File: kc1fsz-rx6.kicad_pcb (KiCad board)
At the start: 2 copper layers, 63.5 x 47.8 mm, 51 parts, among them J1 Conn_Coaxial, J2 Conn_01x07, J3 Conn_01x02, J4 Conn_01x02, U1 SN74CBT3253, U2 LM4562, U3 LM4562

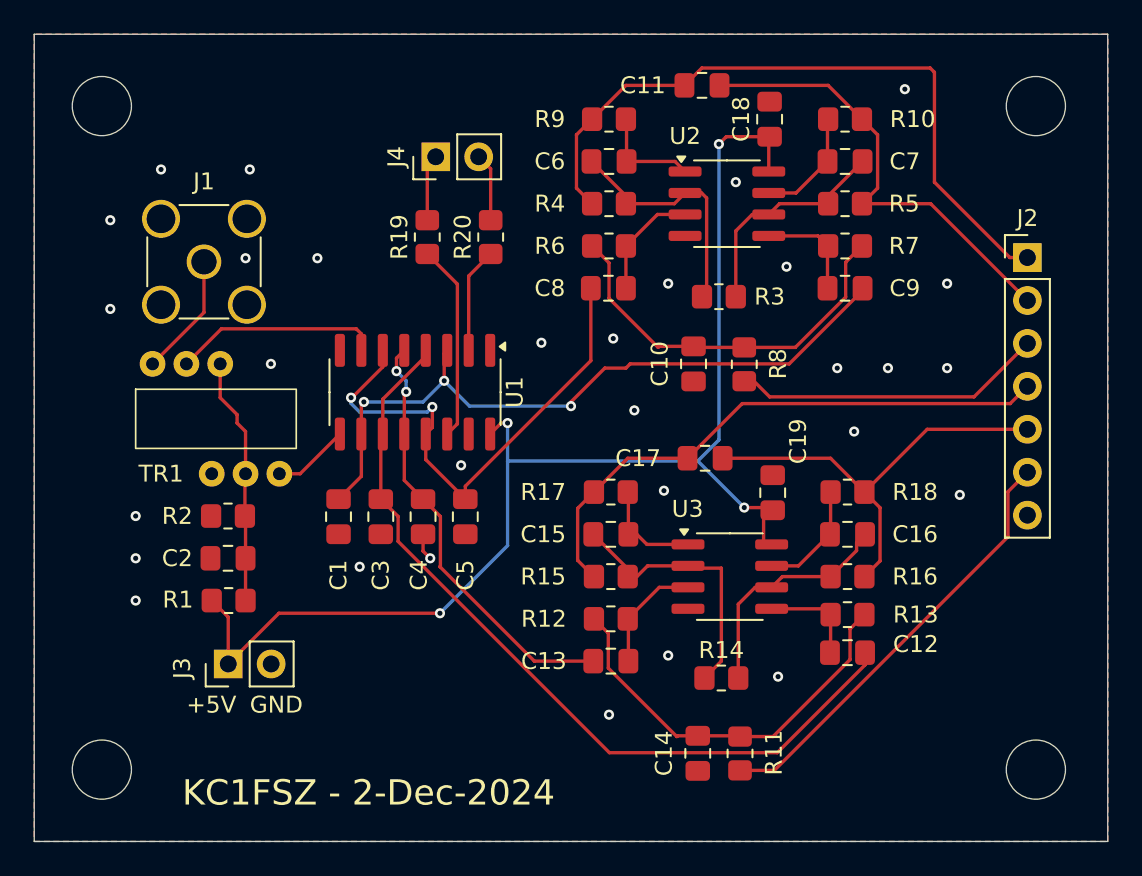
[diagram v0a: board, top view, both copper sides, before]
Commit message: Layout complete
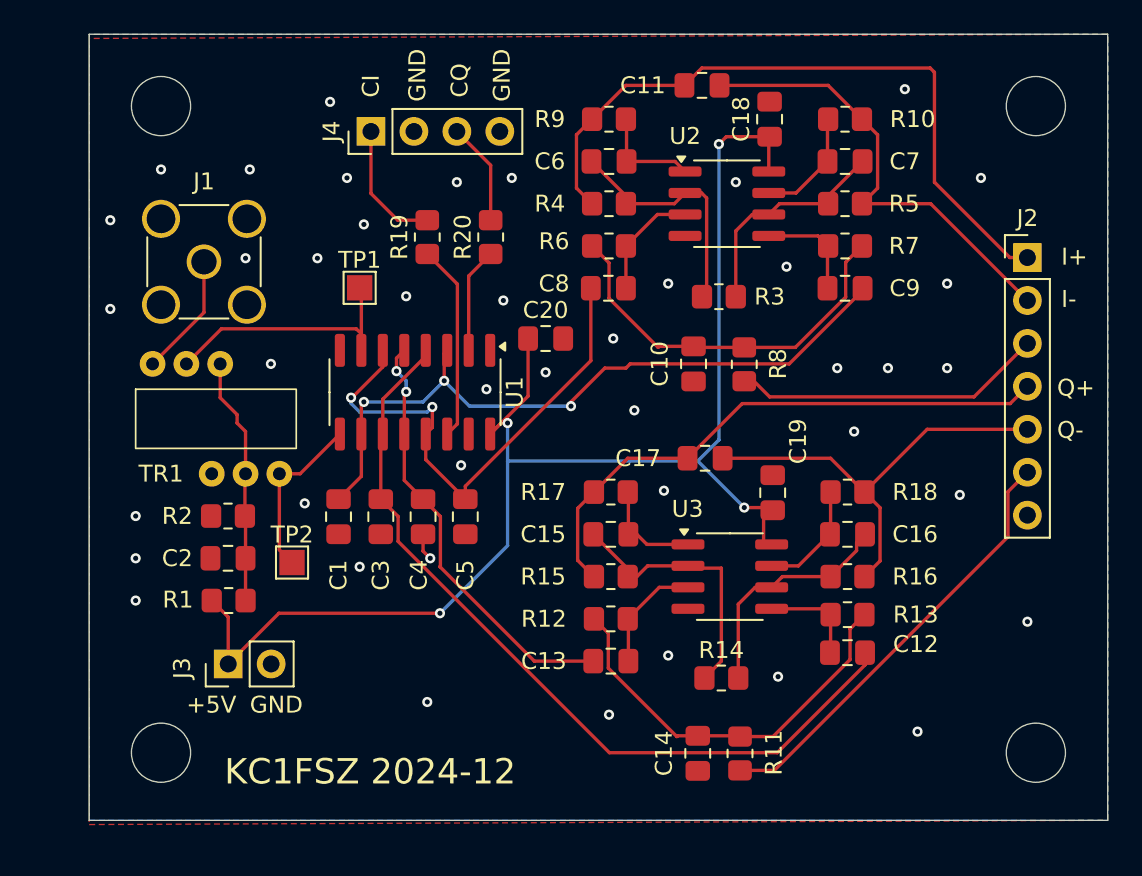
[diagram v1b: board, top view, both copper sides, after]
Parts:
- added C20: 0.1u, Capacitor_SMD:C_0805_2012Metric_Pad1.18x1.45mm_HandSolder, F.Cu at (146.8, 81.0)
- added TP1: TestPoint, TestPoint:TestPoint_Pad_1.5x1.5mm, F.Cu at (135.8, 78.0)
- added TP2: TestPoint, TestPoint:TestPoint_Pad_1.5x1.5mm, F.Cu at (131.8, 94.2)
- J3: value Conn_01x02 -> Power
- J4: value Conn_01x02 -> Clock; footprint Connector_PinHeader_2.54mm:PinHeader_1x02_P2.54mm_Vertical -> Connector_PinHeader_2.54mm:PinHeader_1x04_P2.54mm_Vertical
- moved J4 4.11 mm to (136.4, 68.8)
- moved H2 3.64 mm to (124.0, 105.5)
- moved H1 3.50 mm to (124.0, 67.2)
- moved H4 1.00 mm to (175.8, 105.5)
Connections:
- J4 pad 2: Net-(J4-Pin_2) -> GND
- R20 pad 2: Net-(J4-Pin_2) -> Net-(J4-Pin_3)
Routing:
- net +5V: track 75.5 -> 82.1 mm
- net Net-(J4-Pin_3): track 0.00 -> 6.08 mm
- net Net-(U1-2A): track 4.55 -> 10.1 mm
- net Net-(J4-Pin_2): track 4.04 -> 0.00 mm
- net Net-(U1-1A): track 12.3 -> 16.1 mm
- net Net-(J4-Pin_1): track 3.96 -> 7.65 mm
- net GND: vias 30 -> 43
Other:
- board size 63.5 x 47.8 mm -> 60.2 x 46.5 mm
- board text added: "CI"
- board text added: "CQ"
- board text added: "I+"
- board text added: "I-"
- board text added: "KC1FSZ 2024-12"
- board text added: "Q+"
- board text added: "Q-"
- board text removed: "KC1FSZ - 2-Dec-2024"
